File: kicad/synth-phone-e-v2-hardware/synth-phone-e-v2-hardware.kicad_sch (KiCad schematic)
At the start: 43 parts, among them J1 AudioJack4, J10 Audio_out_input, J11 mic_gain_input, J13 Audio_in_output, J14 Audio_out_output, J15 encoder_input, J2 AudioJack4, J3 DIN-5, J4 Keypad_column_output, J5 Conn_01x04_Pin, J6 USB_C_Receptacle_USB2.0, J7 Conn_01x03_Socket, J8 Conn_01x03_Pin, J9 Audio_IN_INPUT, SW1 SW_Push, SW10 SW_Push, SW11 SW_Push, SW12 SW_Push, SW2 SW_Push, SW3 SW_Push, SW4 SW_Push, SW5 SW_Push, SW6 SW_Push, SW7 SW_Push, SW8 SW_Push, SW9 SW_Push, U1 LM358

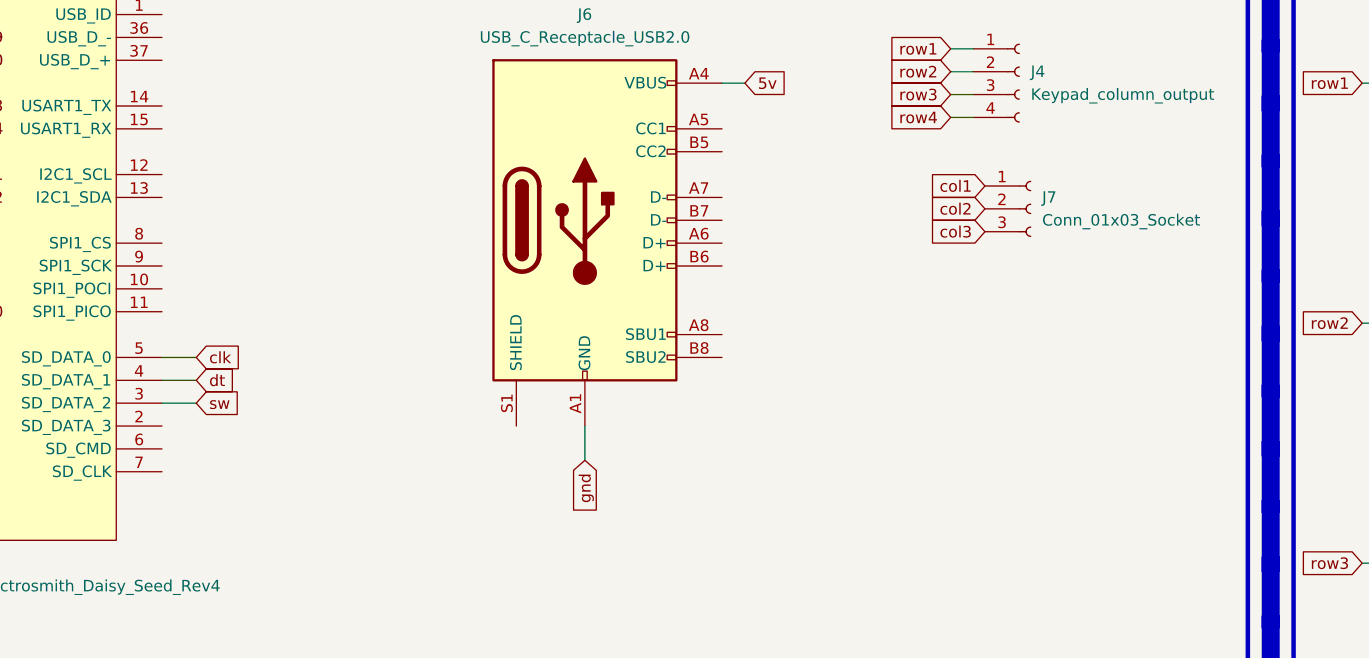
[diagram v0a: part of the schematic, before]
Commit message: feat: basic lcd
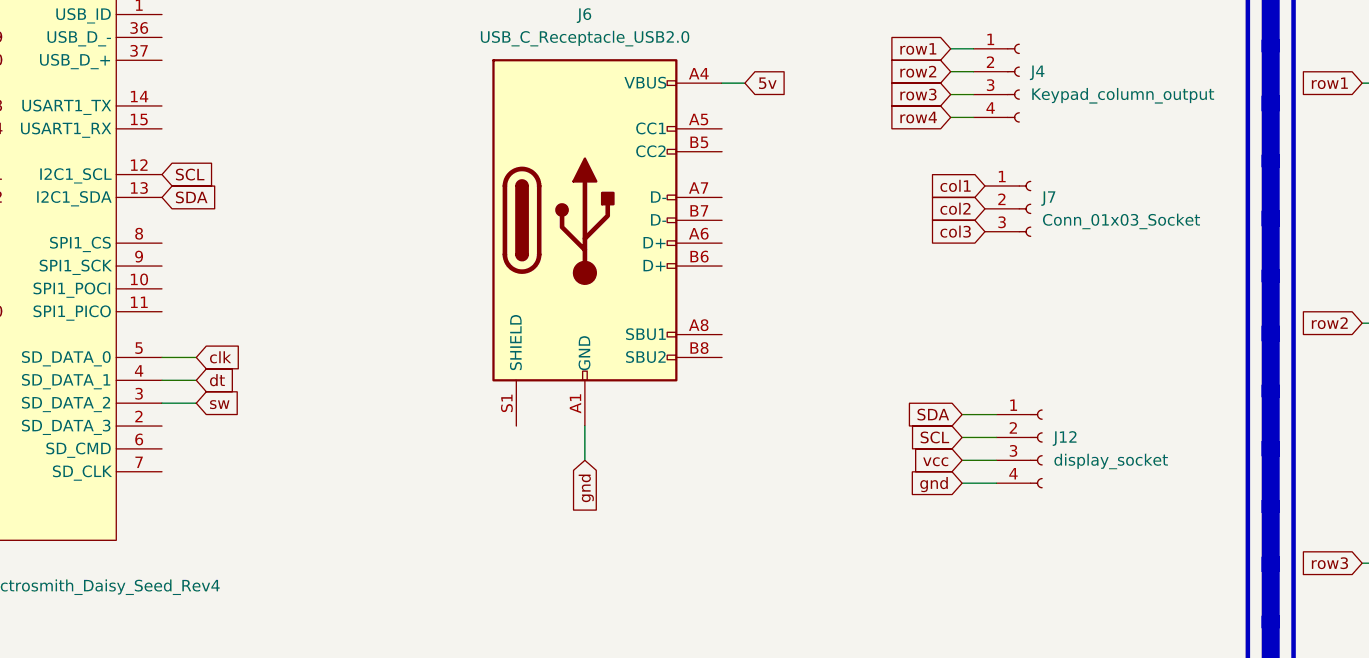
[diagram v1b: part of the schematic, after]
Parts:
- added J12: display_socket, symbol Connector:Conn_01x04_Socket
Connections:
- net gnd: now also J12.4 (Pin_4)
- net vcc: now also J12.3 (Pin_3)
- net SCL: now reaches A1.12 (I2C1_SCL)
- net SCL: now also J12.2 (Pin_2)
- net SDA: now reaches A1.13 (I2C1_SDA)
- net SDA: now also J12.1 (Pin_1)

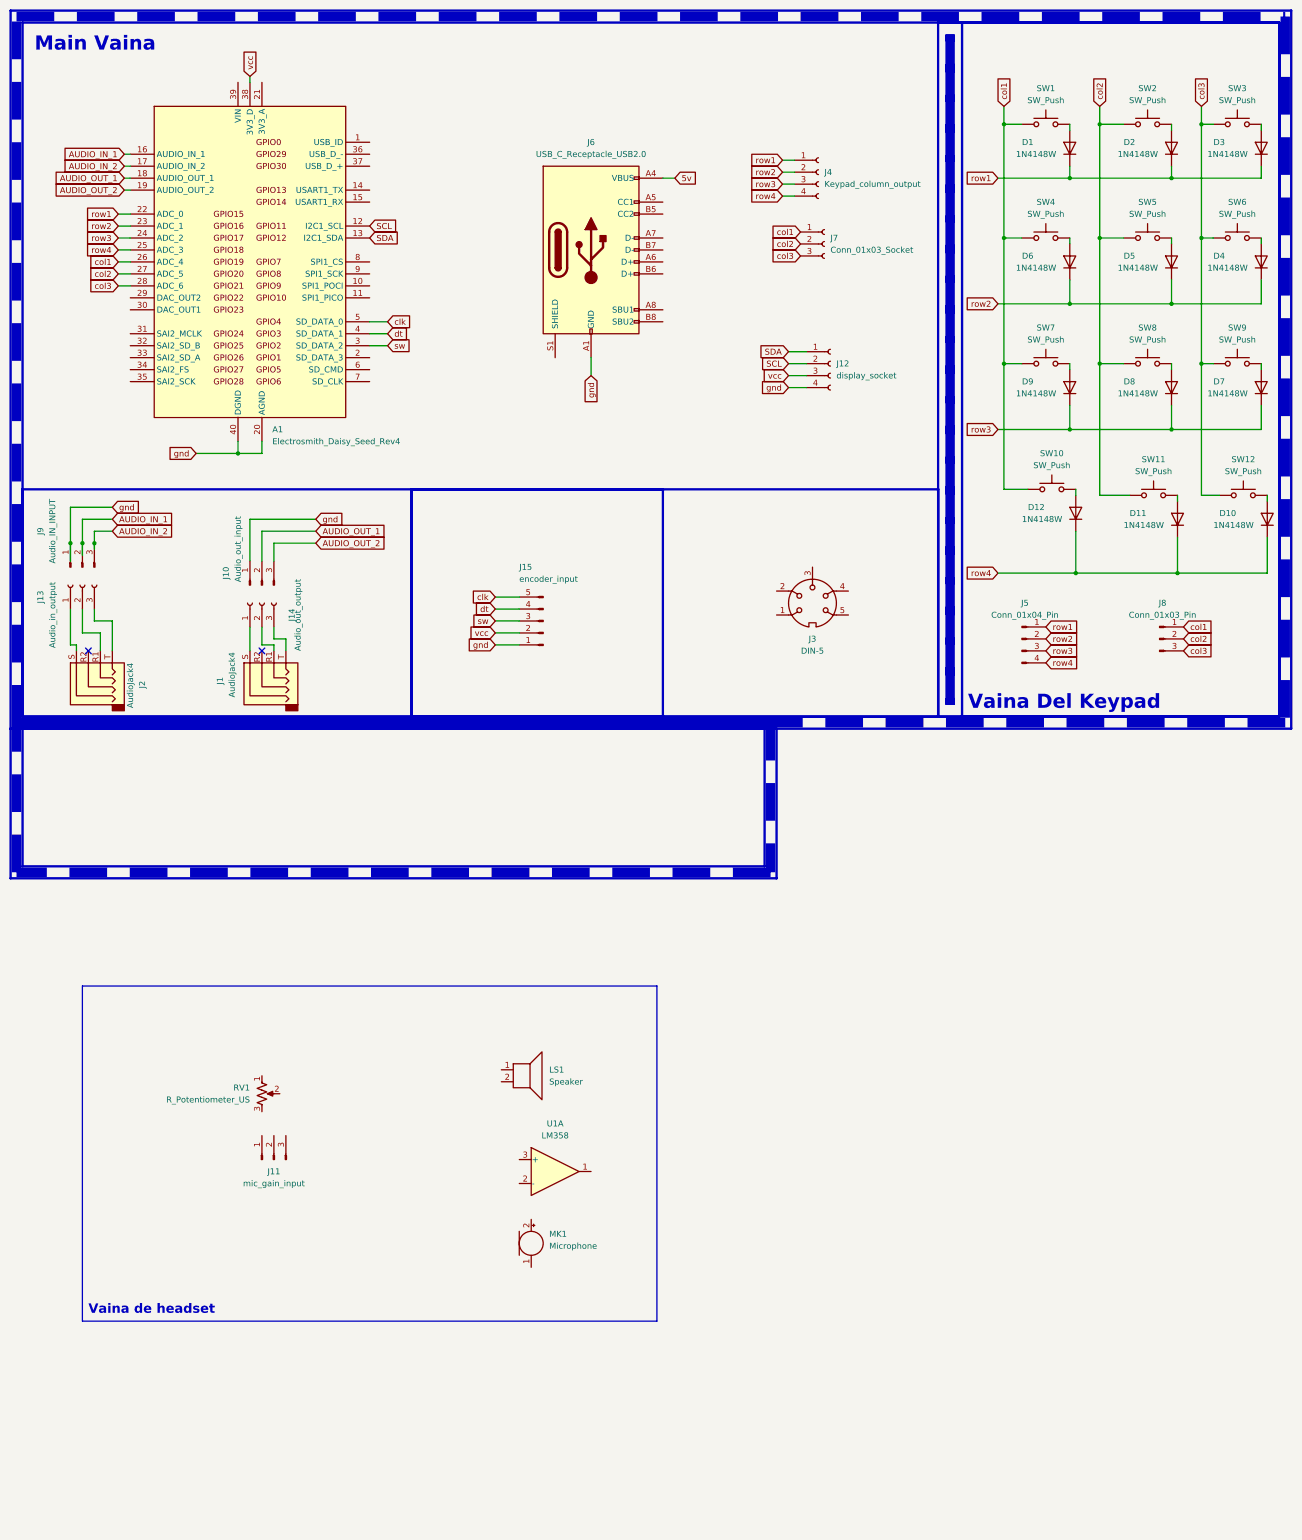
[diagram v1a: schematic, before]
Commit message: chore: update schematic
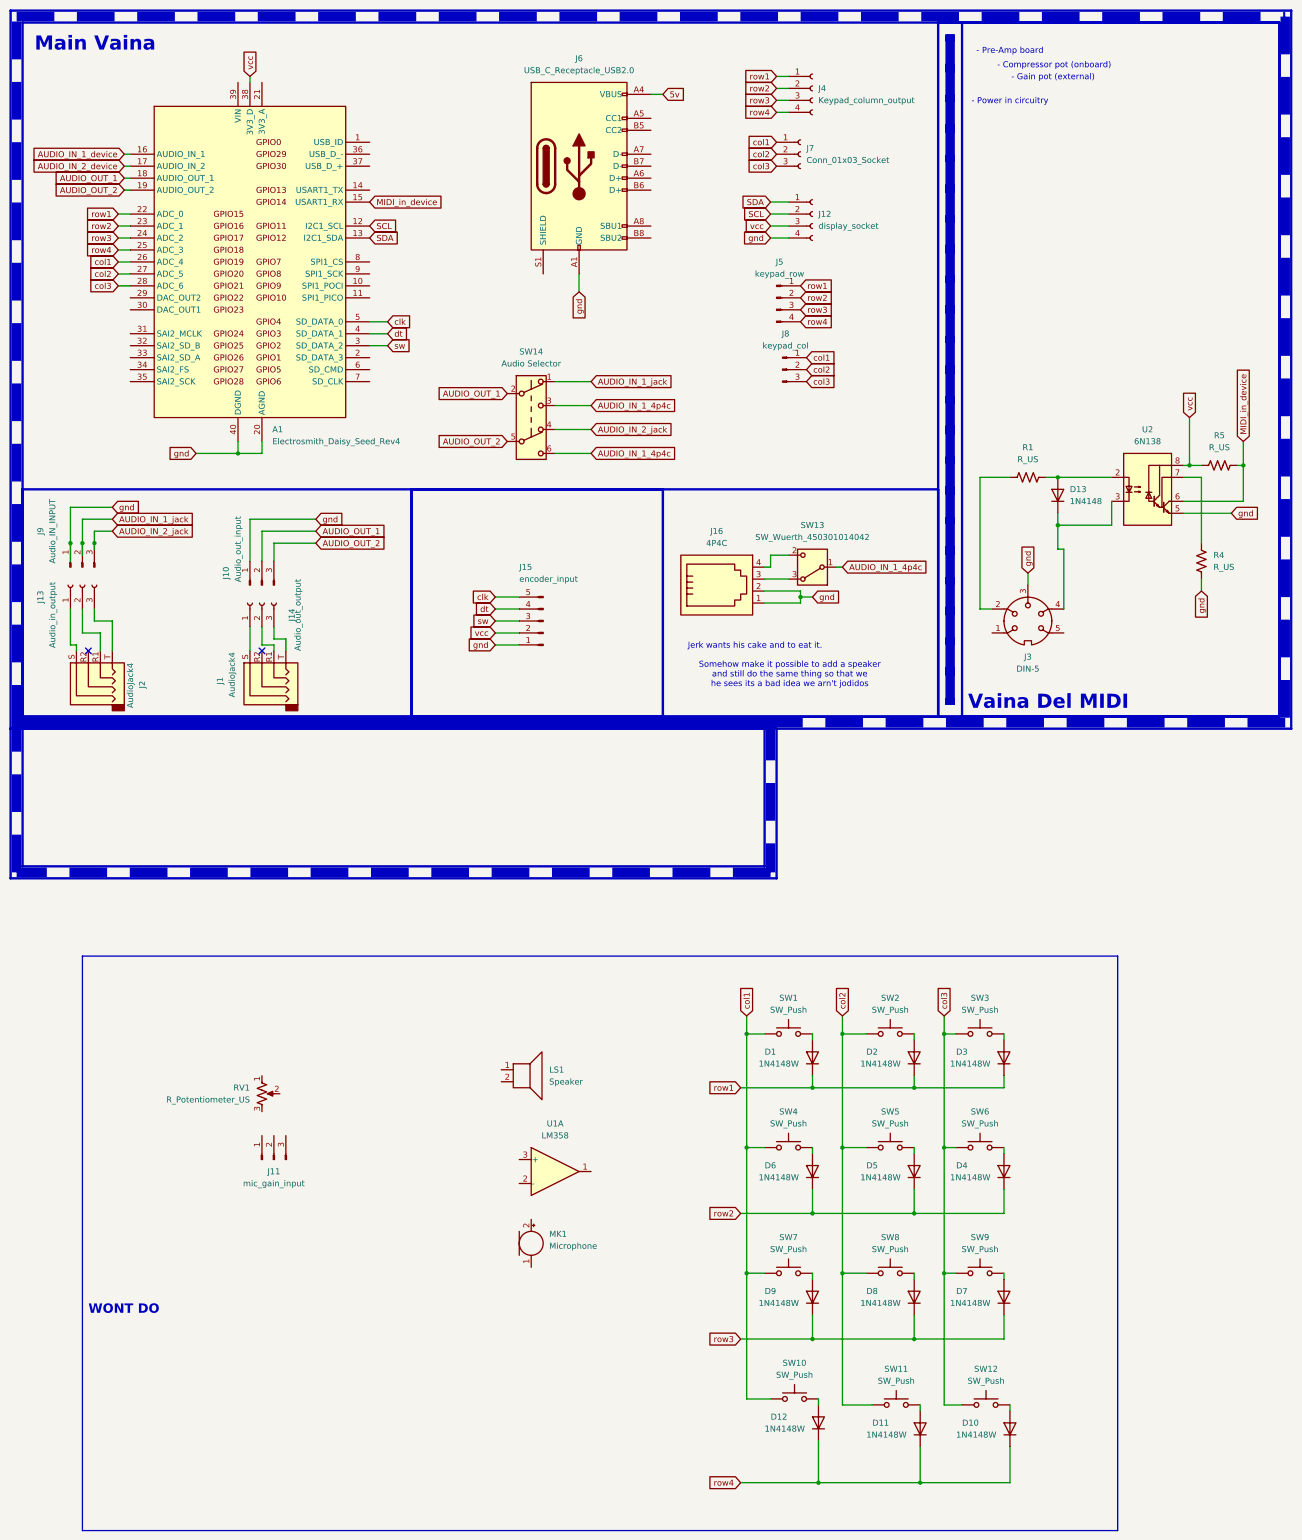
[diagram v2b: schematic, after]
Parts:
- added D13: 1N4148, Diode_THT:D_DO-35_SOD27_P7.62mm_Horizontal, symbol Diode:1N4148
- added J16: 4P4C, symbol Connector:4P4C
- added R1, R4, R5: R_US, symbol Device:R_US
- added SW13: SW_Wuerth_450301014042, Button_Switch_THT:SW_Slide-03_Wuerth-WS-SLTV_10x2.5x6.4_P2.54mm, symbol Switch:SW_Wuerth_450301014042
- added SW14: Audio Selector, symbol Switch:SW_Push_DPDT
- added U2: 6N138, symbol Isolator:6N138
- J5: value Conn_01x04_Pin -> keypad_row
- J8: value Conn_01x03_Pin -> keypad_col
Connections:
- net AUDIO_OUT_1: now also SW14.2 (B)
- net AUDIO_OUT_2: now also SW14.5 (B)
- net gnd: now also J3.3, J16.1, J16.2, R4.1, U2.5 (GND)
- net vcc: now also R5.2, U2.8 (VCC)
- net at J3.2: now also R1.1
- net at J3.4: now also D13.1 (K), U2.3 (C2)
- net MIDI_in_device: now reaches A1.15 (USART1_RX)
- net MIDI_in_device: now also R5.1, U2.6 (VO2)
- net AUDIO_IN_1 renamed AUDIO_IN_1_device
- net AUDIO_IN_1_device: no longer J9.2 (Pin_2)
- net AUDIO_IN_2 renamed AUDIO_IN_2_device
- net AUDIO_IN_2_device: no longer J9.3 (Pin_3)
- new net: R4.2, U2.7 (VO1)
- new net: J16.3, SW13.3 (A)
- new net: J16.4, SW13.2 (C)
- new net: D13.2 (A), R1.2, U2.2 (C1)
- new net AUDIO_IN_1_4p4c: SW13.1 (B), SW14.3 (C), SW14.6 (C)
- new net AUDIO_IN_1_jack: J9.2 (Pin_2), SW14.1 (A)
- new net AUDIO_IN_2_jack: J9.3 (Pin_3), SW14.4 (A)
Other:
- note added: "- Compressor pot (onboard)"
- note added: "- Gain pot (external)"
- note added: "- Power in circuitry"
- note added: "- Pre-Amp board"
- note added: "Jerk wants his cake and to eat it."
- note added: "Somehow make it possible to add a speaker and still do the same thing so that we he sees its a bad idea we arn't jodidos"
- note added: "Vaina Del MIDI"
- note added: "WONT DO"
- note removed: "Vaina Del Keypad"
- note removed: "Vaina de headset"
- moved on the sheet: D1, D10, D11, D12, D2, D3, D4, D5, D6, D7, D8, D9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
